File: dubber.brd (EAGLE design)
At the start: 48.2 x 56.8 mm, 31 parts, among them IC1 LM324N, P1-G TPSQPAD1-13Y, P1-S TPSQPAD1-13Y, P2-G TPSQPAD1-13Y, P2-S TPSQPAD1-13Y, P3-G TPSQPAD1-13Y, P3-S TPSQPAD1-13Y

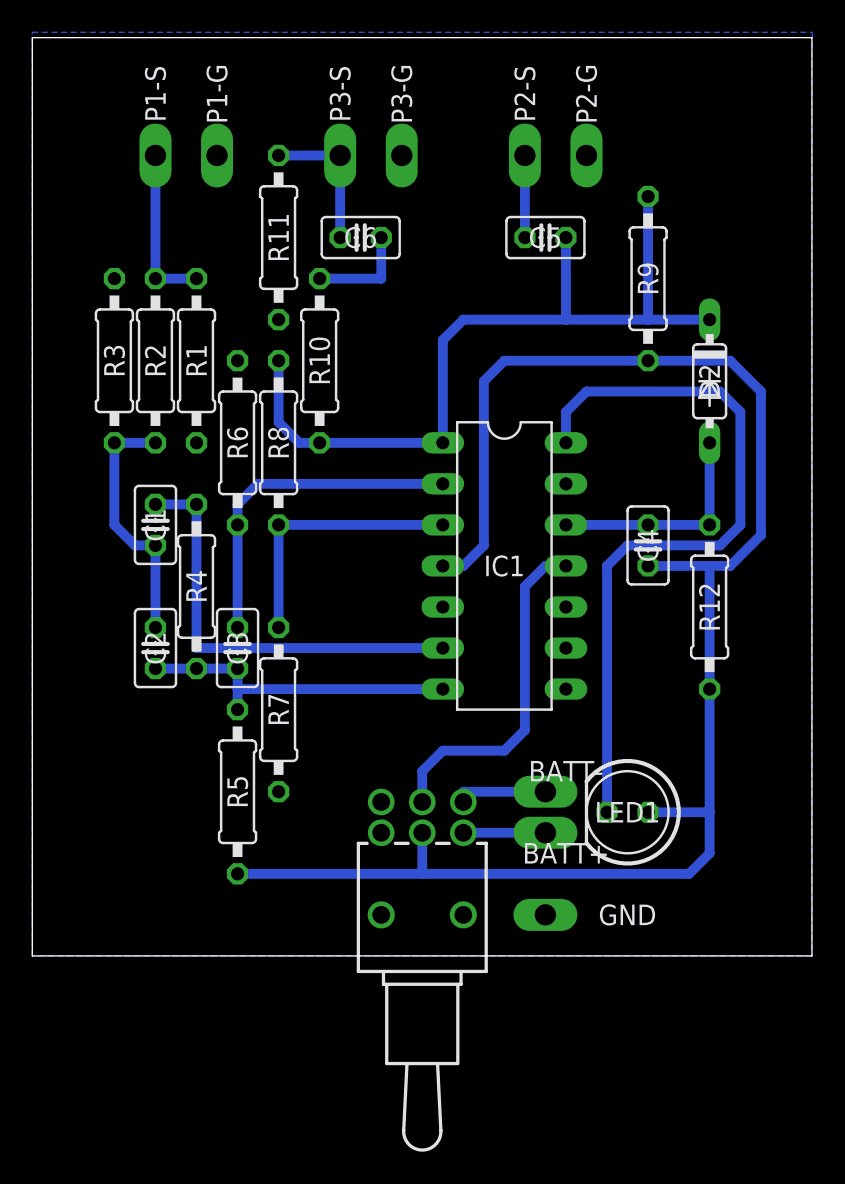
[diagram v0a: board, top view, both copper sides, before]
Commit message: tweaks again
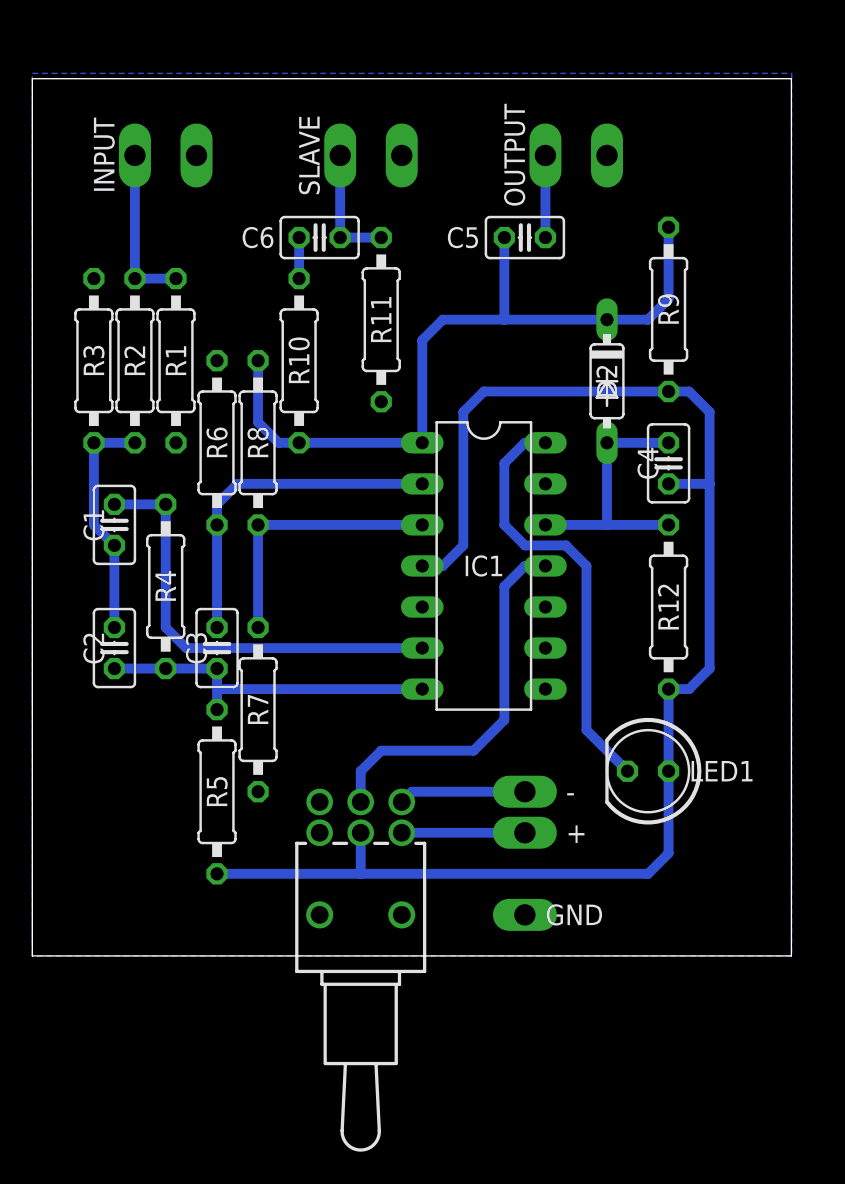
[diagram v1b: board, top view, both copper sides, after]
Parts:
- removed BATT+, BATT-, P1-S, P2-S: TPSQPAD1-13Y, testpad:P1-13Y
- added +, -, INPUT, OUTPUT: TPSQPAD1-13Y, testpad:P1-13Y
- moved R11 8.13 mm to (21.6, 39.4)
- moved D2 6.35 mm to (35.6, 35.6)
- moved C4 5.24 mm to (39.4, 30.5)
- moved S1 3.81 mm to (20.3, 2.54)
- moved LED1 2.84 mm to (38.1, 11.4)
- moved C1 2.54 mm to (5.08, 26.7)
- moved C2 2.54 mm to (5.08, 19.1)
- moved C6 2.54 mm to (17.8, 44.5), turned to 0 degrees
- moved R12 2.54 mm to (39.4, 21.6)
- moved R9 2.29 mm to (39.4, 40.0)
- moved R4 1.90 mm to (8.26, 22.9)
- moved P2-G 1.27 mm to (35.6, 49.5)
- moved R2 1.27 mm to (6.35, 36.8)
- moved R3 1.27 mm to (3.81, 36.8)
- moved C3 1.27 mm to (11.4, 19.1)
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- renumbered P3-S to SLAVE
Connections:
- net N$14: now also OUTPUT.TP; no longer P2-S.TP
- net N$17: now also INPUT.TP; no longer P1-S.TP
- net N$4: now also +.TP; no longer BATT+.TP
- net N$5: now also -.TP; no longer BATT-.TP
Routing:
- net N$12: track 45.3 -> 26.8 mm
- net V+: track 102.2 -> 90.3 mm
- net N$10: track 50.6 -> 46.7 mm
- net N$3: track 6.35 -> 2.54 mm
- net N$4: track 5.08 -> 7.62 mm
- net N$9: track 14.0 -> 16.5 mm
- net N$5: track 5.71 -> 7.88 mm
- net V-: track 21.3 -> 23.4 mm
- net N$21: track 8.89 -> 7.62 mm
- net N$2: track 20.3 -> 21.6 mm
- net N$1: track 15.8 -> 14.5 mm
- net N$16: track 26.7 -> 27.2 mm
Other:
- board size 48.2 x 56.8 mm -> 47 x 54.3 mm
